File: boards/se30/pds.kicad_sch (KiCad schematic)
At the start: 1 part, among them J1 Mac SE/30 PDS Interface

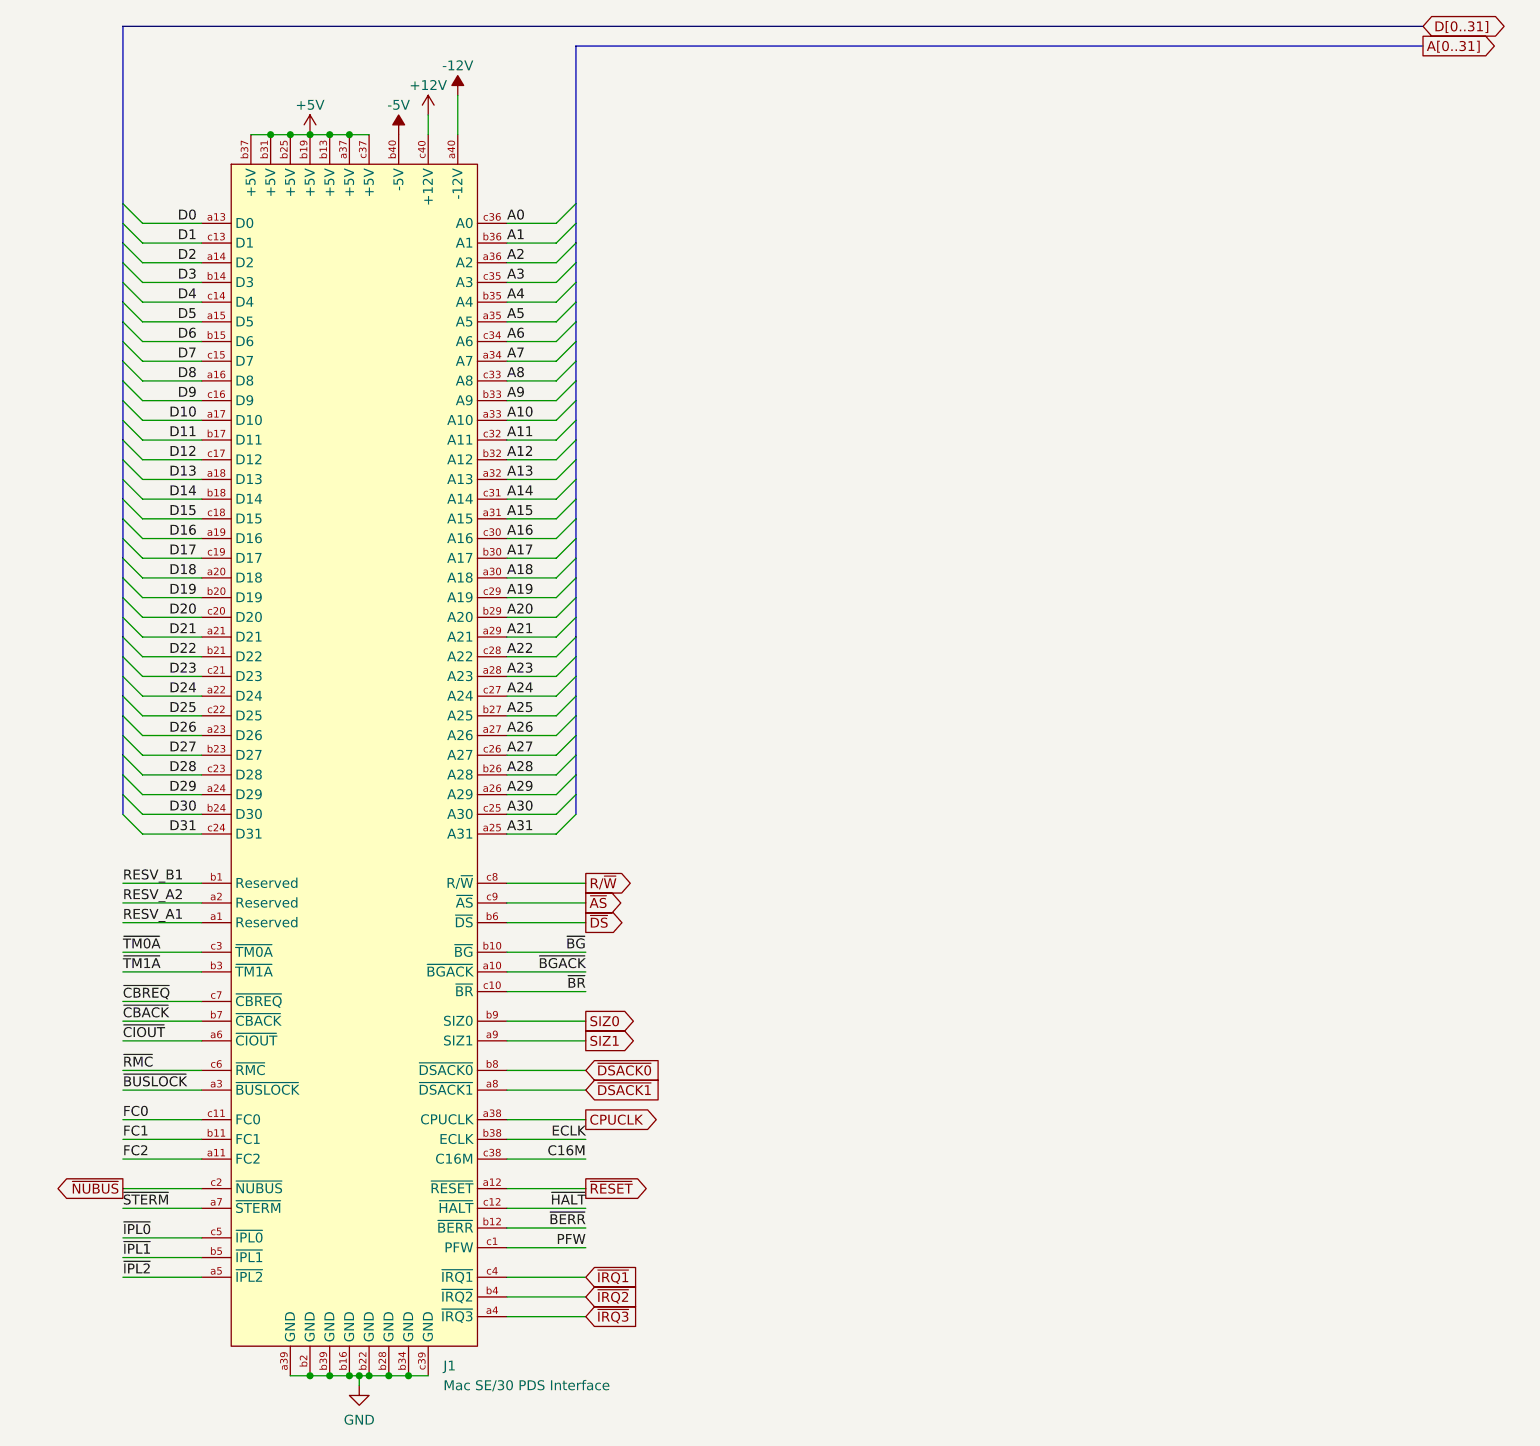
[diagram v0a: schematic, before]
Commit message: Rev1 hardware
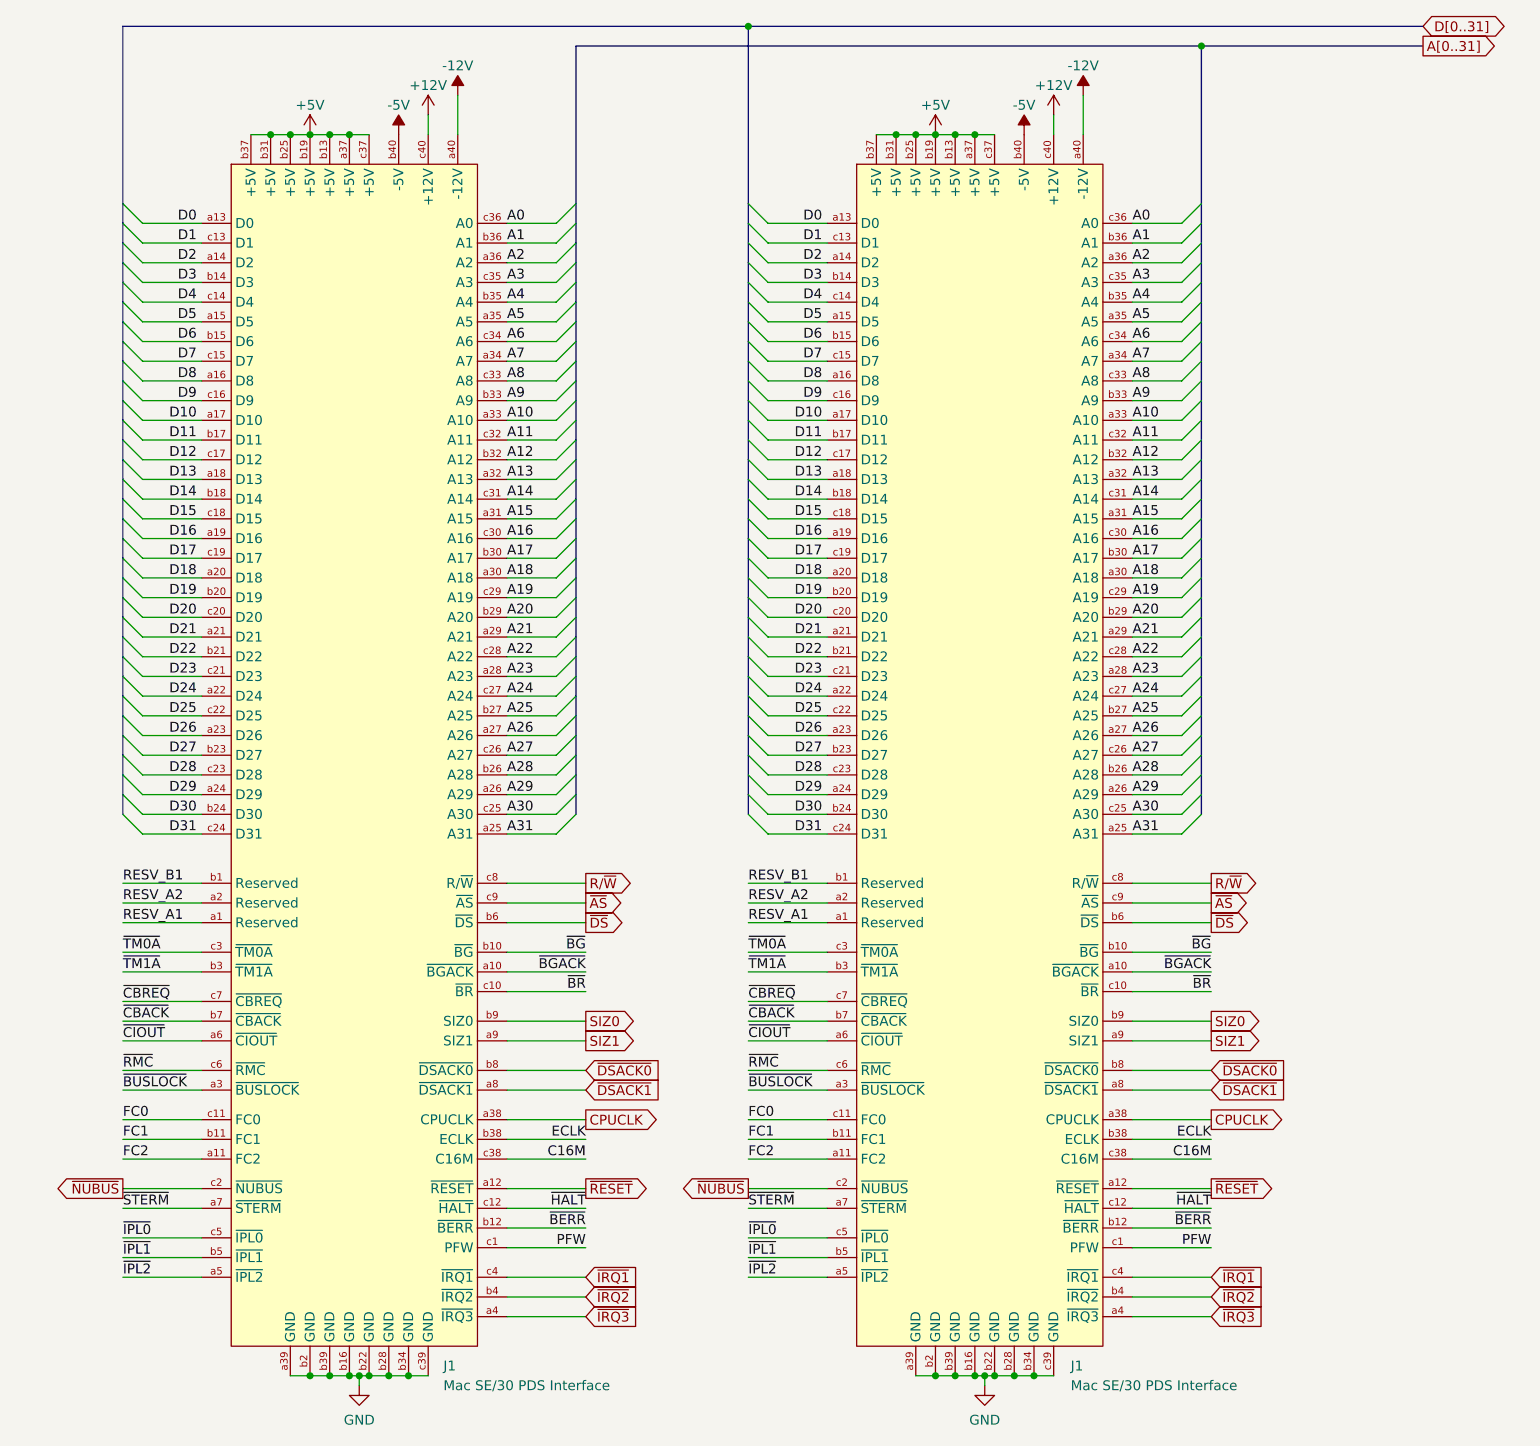
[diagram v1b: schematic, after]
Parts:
- added J1: Mac SE/30 PDS Interface, PDS-Ethernet:DIN41612_C_3x40_Female_Horizontal_THT, symbol PDS-Ethernet:SE30_PDS
- J1: Digikey 650906-5 -> A124347-ND; LCSC (none) -> C3652939
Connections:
- net +12V: now also J1.c40 (+12V)
- net +5V: now also J1.a37 (+5V), J1.b13 (+5V), J1.b19 (+5V), J1.b25 (+5V), J1.b31 (+5V), J1.b37 (+5V), J1.c37 (+5V)
- net -12V: now also J1.a40 (-12V)
- net -5V: now also J1.b40 (-5V)
- net A0: now also J1.c36 (A0)
- net A1: now also J1.b36 (A1)
- net A10: now also J1.a33 (A10)
- net A11: now also J1.c32 (A11)
- net A12: now also J1.b32 (A12)
- net A13: now also J1.a32 (A13)
- net A14: now also J1.c31 (A14)
- net A15: now also J1.a31 (A15)
- net A16: now also J1.c30 (A16)
- net A17: now also J1.b30 (A17)
- net A18: now also J1.a30 (A18)
- net A19: now also J1.c29 (A19)
- net A2: now also J1.a36 (A2)
- net A20: now also J1.b29 (A20)
- net A21: now also J1.a29 (A21)
- net A22: now also J1.c28 (A22)
- net A23: now also J1.a28 (A23)
- net A24: now also J1.c27 (A24)
- net A25: now also J1.b27 (A25)
- net A26: now also J1.a27 (A26)
- net A27: now also J1.c26 (A27)
- net A28: now also J1.b26 (A28)
- net A29: now also J1.a26 (A29)
- net A3: now also J1.c35 (A3)
- net A30: now also J1.c25 (A30)
- net A31: now also J1.a25 (A31)
- net A4: now also J1.b35 (A4)
- net A5: now also J1.a35 (A5)
- net A6: now also J1.c34 (A6)
- net A7: now also J1.a34 (A7)
- net A8: now also J1.c33 (A8)
- net A9: now also J1.b33 (A9)
- net C16M: now also J1.c38 (C16M)
- net CPUCLK: now also J1.a38 (CPUCLK)
- net D0: now also J1.a13 (D0)
- net D1: now also J1.c13 (D1)
- net D10: now also J1.a17 (D10)
- net D11: now also J1.b17 (D11)
- net D12: now also J1.c17 (D12)
- net D13: now also J1.a18 (D13)
- net D14: now also J1.b18 (D14)
- net D15: now also J1.c18 (D15)
- net D16: now also J1.a19 (D16)
- net D17: now also J1.c19 (D17)
- net D18: now also J1.a20 (D18)
- net D19: now also J1.b20 (D19)
- net D2: now also J1.a14 (D2)
- net D20: now also J1.c20 (D20)
- net D21: now also J1.a21 (D21)
- net D22: now also J1.b21 (D22)
- net D23: now also J1.c21 (D23)
- net D24: now also J1.a22 (D24)
- net D25: now also J1.c22 (D25)
- net D26: now also J1.a23 (D26)
- net D27: now also J1.b23 (D27)
- net D28: now also J1.c23 (D28)
- net D29: now also J1.a24 (D29)
- net D3: now also J1.b14 (D3)
- net D30: now also J1.b24 (D30)
- net D31: now also J1.c24 (D31)
- net D4: now also J1.c14 (D4)
- net D5: now also J1.a15 (D5)
- net D6: now also J1.b15 (D6)
- net D7: now also J1.c15 (D7)
- net D8: now also J1.a16 (D8)
- net D9: now also J1.c16 (D9)
- net ECLK: now also J1.b38 (ECLK)
- net FC0: now also J1.c11 (FC0)
- net FC1: now also J1.b11 (FC1)
- net FC2: now also J1.a11 (FC2)
- net GND: now also J1.a39 (GND), J1.b16 (GND), J1.b2 (GND), J1.b22 (GND), J1.b28 (GND), J1.b34 (GND), J1.b39 (GND), J1.c39 (GND)
- net PFW: now also J1.c1 (PFW)
- net RESV_A1: now also J1.a1 (Reserved)
- net RESV_A2: now also J1.a2 (Reserved)
- net RESV_B1: now also J1.b1 (Reserved)
- net R/~{W}: now also J1.c8 (R/~{W})
- net SIZ0: now also J1.b9 (SIZ0)
- net SIZ1: now also J1.a9 (SIZ1)
- net ~{AS}: now also J1.c9 (~{AS})
- net ~{BERR}: now also J1.b12 (~{BERR})
- net ~{BGACK}: now also J1.a10 (~{BGACK})
- net ~{BG}: now also J1.b10 (~{BG})
- net ~{BR}: now also J1.c10 (~{BR})
- net ~{BUSLOCK}: now also J1.a3 (~{BUSLOCK})
- net ~{CBACK}: now also J1.b7 (~{CBACK})
- net ~{CBREQ}: now also J1.c7 (~{CBREQ})
- net ~{CIOUT}: now also J1.a6 (~{CIOUT})
- net ~{DSACK0}: now also J1.b8 (~{DSACK0})
- net ~{DSACK1}: now also J1.a8 (~{DSACK1})
- net ~{DS}: now also J1.b6 (~{DS})
- net ~{HALT}: now also J1.c12 (~{HALT})
- net ~{IPL0}: now also J1.c5 (~{IPL0})
- net ~{IPL1}: now also J1.b5 (~{IPL1})
- net ~{IPL2}: now also J1.a5 (~{IPL2})
- net ~{IRQ1}: now also J1.c4 (~{IRQ1})
- net ~{IRQ2}: now also J1.b4 (~{IRQ2})
- net ~{IRQ3}: now also J1.a4 (~{IRQ3})
- net ~{NUBUS}: now also J1.c2 (~{NUBUS})
- net ~{RESET}: now also J1.a12 (~{RESET})
- net ~{RMC}: now also J1.c6 (~{RMC})
- net ~{STERM}: now also J1.a7 (~{STERM})
- net ~{TM0A}: now also J1.c3 (~{TM0A})
- net ~{TM1A}: now also J1.b3 (~{TM1A})
